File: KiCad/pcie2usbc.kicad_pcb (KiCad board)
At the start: 4 copper layers, 64.5 x 37.3 mm, 70 parts, among them J1 Bus_PCI_Express_x4, J2 Conn_02x05_Top_Bottom, J3 USB-C-MLX, J4 USB-C-MLX

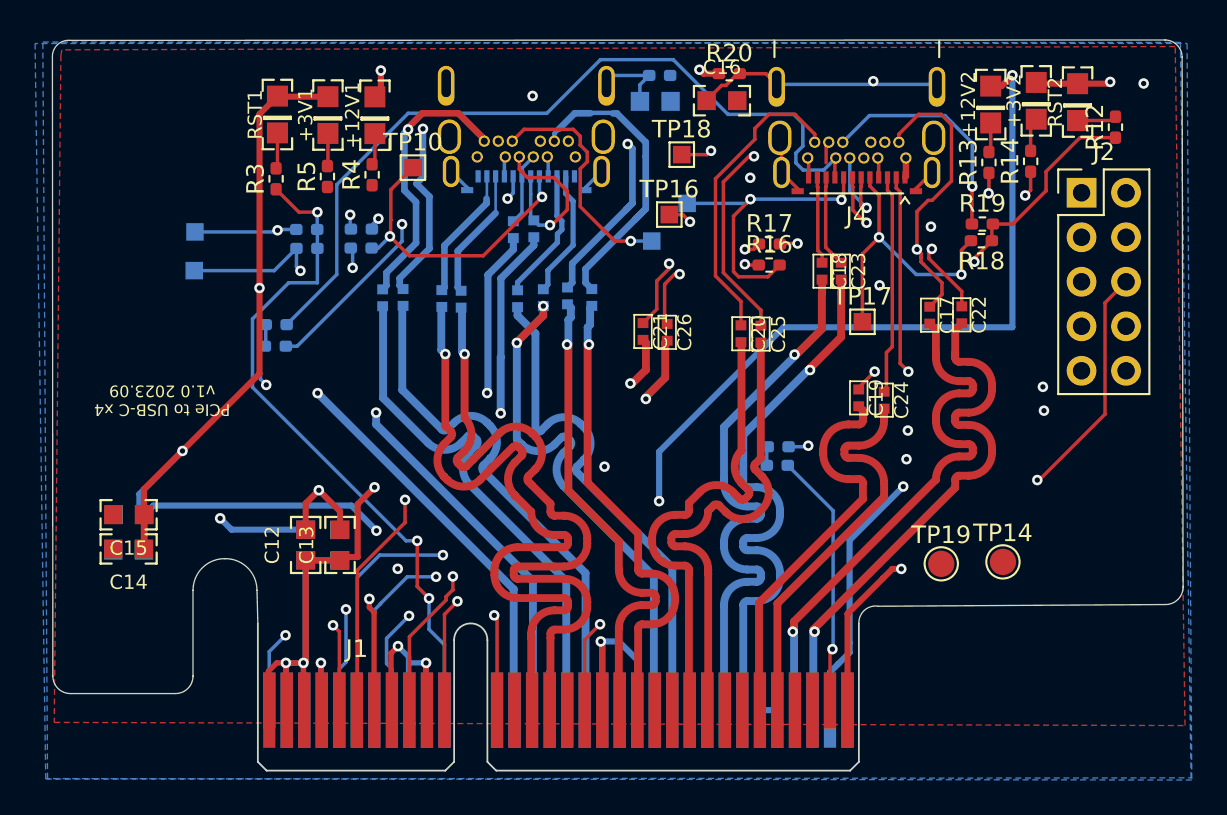
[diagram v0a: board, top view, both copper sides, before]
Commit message: Final rework
Layout completed finally
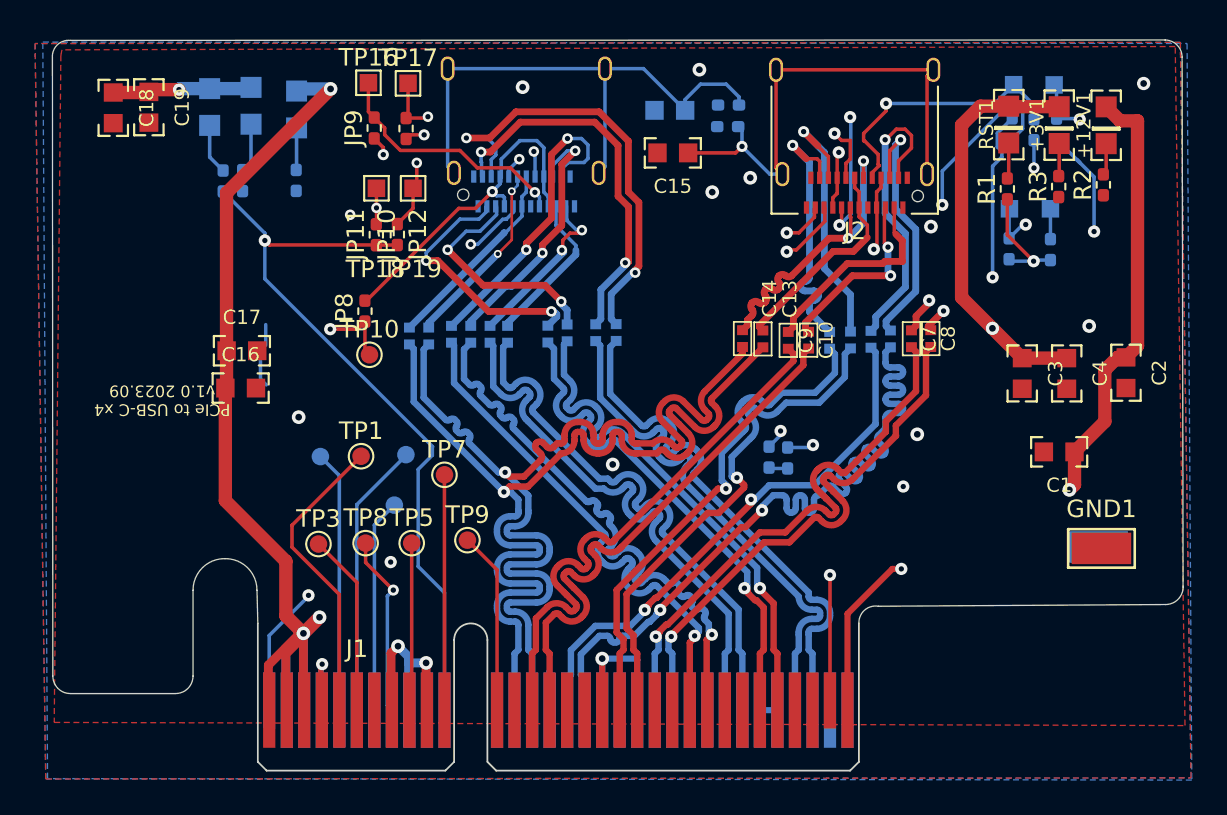
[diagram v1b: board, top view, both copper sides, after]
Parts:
- removed J4: USB-C-MLX, Connector_USB:USB_C_Receptacle_CNCTech_C-ARA1-AK51X
- removed R16, R17, R18, R19: 0, Resistor_SMD:R_0402_1005Metric_Pad0.72x0.64mm_HandSolder
- removed R20: 100k, Resistor_SMD:R_0402_1005Metric_Pad0.72x0.64mm_HandSolder
- added GND1: TestPoint, TestPoint:TestPoint_Keystone_5015_Micro-Minature, F.Cu at (190.7, 104.2)
- added JP3: 0, Resistor_SMD:R_0402_1005Metric_Pad0.72x0.64mm_HandSolder, B.Cu at (185.6, 80.3)
- added JP4: 0, Resistor_SMD:R_0402_1005Metric_Pad0.72x0.64mm_HandSolder, B.Cu at (188.1, 80.3)
- added JP5: 0, Resistor_SMD:R_0402_1005Metric_Pad0.72x0.64mm_HandSolder, B.Cu at (186.8, 80.3)
- added JP6: 0, Resistor_SMD:R_0402_1005Metric_Pad0.72x0.64mm_HandSolder, B.Cu at (187.8, 87.2)
- added JP7: 0, Resistor_SMD:R_0402_1005Metric_Pad0.72x0.64mm_HandSolder, B.Cu at (185.4, 87.1)
- added TP1: TestPoint_Small, TestPoint:TestPoint_Pad_D1.0mm, F.Cu at (148.4, 99.0)
- added TP2: TestPoint_Small, TestPoint:TestPoint_Pad_D1.0mm, B.Cu at (146.1, 99.0)
- added TP3: TestPoint_Small, TestPoint:TestPoint_Pad_D1.0mm, F.Cu at (146.0, 104.0)
- added TP4: TestPoint_Small, TestPoint:TestPoint_Pad_D1.0mm, B.Cu at (151.0, 98.9)
- added TP5: TestPoint_Small, TestPoint:TestPoint_Pad_D1.0mm, F.Cu at (151.3, 103.9)
- added TP6: TestPoint_Small, TestPoint:TestPoint_Pad_D1.0mm, B.Cu at (150.3, 101.8)
- added TP7: TestPoint_Small, TestPoint:TestPoint_Pad_D1.0mm, F.Cu at (153.2, 100.0)
- added TP8: TestPoint_Small, TestPoint:TestPoint_Pad_D1.0mm, F.Cu at (148.7, 103.9)
- added TP9: TestPoint_Small, TestPoint:TestPoint_Pad_D1.0mm, F.Cu at (154.5, 103.8)
- +12V2, +3V2, C20, C21, C22, C23, C24, C25, C26, RST2: moved to B.Cu
- C1: value 100n -> 1u; moved to F.Cu
- C10, C7, C8, C9: moved to F.Cu
- C12: value 1u -> 100n; footprint pcie2usbc:C0603K -> pcie2usbc:C0402; moved to B.Cu
- C13, C28: footprint pcie2usbc:C0603K -> pcie2usbc:C0402
- C14, C27, C29: value 1u -> 100n; footprint pcie2usbc:C0603K -> pcie2usbc:C0402
- C16: value 100n -> 1u
- C17, C19: footprint pcie2usbc:C0402 -> pcie2usbc:C0603K
- C18: value 100n -> 1u; footprint pcie2usbc:C0402 -> pcie2usbc:C0603K
- C2, C4: footprint pcie2usbc:C0402 -> pcie2usbc:C0603K; moved to F.Cu
- C3: value 100n -> 1u; footprint pcie2usbc:C0402 -> pcie2usbc:C0603K; moved to F.Cu
- J2: value Conn_02x05_Top_Bottom -> USB-C-MLX; footprint Connector_PinHeader_2.54mm:PinHeader_2x05_P2.54mm_Vertical -> Connector_USB:USB_C_Receptacle_Amphenol_12401610E4-2A
- J3: footprint Connector_USB:USB_C_Receptacle_CNCTech_C-ARA1-AK51X -> Connector_USB:USB_C_Receptacle_Amphenol_12401610E4-2A
- JP10: renamed from R12; value 2.2k -> 0
- JP11: renamed from R13; value 10k -> 0
- JP12: renamed from R14; value 2.2k -> 0
- JP8: renamed from R10; moved to F.Cu
- JP9: renamed from R11; value 100k -> 0; moved to F.Cu
- R4: renamed from R6; value 0 -> 100k
- R5: renamed from R7; value 0 -> 2.2k
- R6: renamed from R8; value 0 -> 10k
- R7: renamed from R9; value 0 -> 2.2k
- R8: renamed from R15; value 0 -> 100k
- TP10: value TestPoint -> TestPoint_Small; footprint TestPoint:TestPoint_Pad_1.0x1.0mm -> TestPoint:TestPoint_Pad_D1.0mm
- TP14: value TPTP38X20 -> TestPoint; footprint TestPoint:TestPoint_Pad_D1.5mm -> TestPoint:TestPoint_Pad_1.0x1.0mm; moved to B.Cu
- TP15: footprint TestPoint:TestPoint_Pad_1.0x1.0mm -> TestPoint:TestPoint_Keystone_5015_Micro-Minature
- TP19: value TPTP38X20 -> TestPoint; footprint TestPoint:TestPoint_Pad_D1.5mm -> TestPoint:TestPoint_Pad_1.0x1.0mm
- moved RST2 49.5 mm to (139.8, 79.0)
- moved TP13 49.0 mm to (187.8, 84.8), turned to -90 degrees
- moved TP12 47.5 mm to (185.7, 77.8), turned to -90 degrees
- moved +3V2 44.8 mm to (142.2, 79.0)
- moved C19 43.8 mm to (136.3, 79.0)
- moved C2 42.6 mm to (192.1, 94.2)
- moved +12V1 41.7 mm to (191.0, 80.1)
- moved R2 41.7 mm to (190.8, 83.5)
- moved RST1 41.7 mm to (185.4, 80.0)
- moved +3V1 41.7 mm to (188.3, 80.1)
- moved R1 41.7 mm to (185.3, 83.7)
- moved R3 41.7 mm to (188.2, 83.6)
- moved C18 41.5 mm to (134.3, 79.1)
- moved JP10 40.5 mm to (151.0, 80.3)
- moved +12V2 39.6 mm to (144.8, 79.2)
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- renumbered R1 to JP1, R2 to JP2, R3 to R1, R4 to R2, R5 to R3
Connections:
- C1 pad 1: Net-(C1-Pad1) -> +12V
- C10 pad 1: /USB-C Lane1+2/TX2_N -> /USB-C Lane1+2/TX1_N
- C10 pad 2: /PET1_N -> /PET0_N
- C11 pad 1: /USB-C Lane1+2/D_N -> /USB-C Lane1+2/TX2_P
- C11 pad 2: /REFCLK_N -> /PET1_P
- C12 pad 1: +12V -> /USB-C Lane1+2/TX2_N
- C12 pad 2: GND -> /PET1_N
- C13 pad 1: +12V -> /USB-C Lane1+2/D_P
- C13 pad 2: GND -> /REFCLK_P
- C14 pad 1: +3V3 -> /USB-C Lane1+2/D_N
- C14 pad 2: GND -> /REFCLK_N
- C15 pad 1: +3V3 -> Net-(J2-SHIELD)
- C16 pad 1: Net-(C16-Pad1) -> +12V
- C17 pad 1: /USB-C Lane3+4/RX1_P -> +12V
- C17 pad 2: /PER3_P -> GND
- C18 pad 1: /USB-C Lane3+4/RX2_P -> +3V3
- C18 pad 2: /PER2_P -> GND
- C19 pad 1: /USB-C Lane3+4/TX1_P -> +3V3
- C19 pad 2: /PET3_P -> GND
- C2 pad 1: /USB-C Lane1+2/RX1_P -> +12V
- C2 pad 2: /PER0_P -> GND
- C20 pad 1: /USB-C Lane3+4/TX2_P -> /USB-C Lane3+4/RX1_P
- C20 pad 2: /PET2_P -> /PER3_P
- C21 pad 1: /USB-C Lane3+4/D_P -> /USB-C Lane3+4/RX1_N
- C21 pad 2: /REFCLK_P -> /PER3_N
- C22 pad 1: /USB-C Lane3+4/RX1_N -> /USB-C Lane3+4/RX2_P
- C22 pad 2: /PER3_N -> /PER2_P
- C24 pad 1: /USB-C Lane3+4/TX1_N -> /USB-C Lane3+4/TX1_P
- C24 pad 2: /PET3_N -> /PET3_P
- C25 pad 1: /USB-C Lane3+4/TX2_N -> /USB-C Lane3+4/TX1_N
- C25 pad 2: /PET2_N -> /PET3_N
- C26 pad 1: /USB-C Lane3+4/D_N -> /USB-C Lane3+4/TX2_P
- C26 pad 2: /REFCLK_N -> /PET2_P
- C27 pad 1: +12V -> /USB-C Lane3+4/TX2_N
- C27 pad 2: GND -> /PET2_N
- C28 pad 1: +12V -> /USB-C Lane3+4/D_P
- C28 pad 2: GND -> /REFCLK_P
- C29 pad 1: +3V3 -> /USB-C Lane3+4/D_N
- C29 pad 2: GND -> /REFCLK_N
- C3 pad 1: /USB-C Lane1+2/RX2_P -> +3V3
- C3 pad 2: /PER1_P -> GND
- C30 pad 1: +3V3 -> Net-(J3-SHIELD)
- C4 pad 1: /USB-C Lane1+2/TX1_P -> +3V3
- C4 pad 2: /PET0_P -> GND
- C5 pad 1: /USB-C Lane1+2/TX2_P -> /USB-C Lane1+2/RX1_P
- C5 pad 2: /PET1_P -> /PER0_P
- C6 pad 1: /USB-C Lane1+2/D_P -> /USB-C Lane1+2/RX1_N
- C6 pad 2: /REFCLK_P -> /PER0_N
- C7 pad 1: /USB-C Lane1+2/RX1_N -> /USB-C Lane1+2/RX2_P
- C7 pad 2: /PER0_N -> /PER1_P
- C9 pad 1: /USB-C Lane1+2/TX1_N -> /USB-C Lane1+2/TX1_P
- C9 pad 2: /PET0_N -> /PET0_P
- J1 pad B17: /PRSNT2 -> unconnected-(J1-~{PRSNT2}-PadB17)
- J3 pad A10: /USB-C Lane1+2/RX2_N -> /USB-C Lane3+4/RX2_N
- J3 pad A11: /USB-C Lane1+2/RX2_P -> /USB-C Lane3+4/RX2_P
- J3 pad A2: /USB-C Lane1+2/TX1_P -> /USB-C Lane3+4/TX1_P
- J3 pad A3: /USB-C Lane1+2/TX1_N -> /USB-C Lane3+4/TX1_N
- J3 pad A4: /USB-C Lane1+2/VBUS -> /USB-C Lane3+4/VBUS
- J3 pad A5: /USB-C Lane1+2/CC1 -> /USB-C Lane3+4/CC1
- J3 pad A6: /USB-C Lane1+2/D_P -> /USB-C Lane3+4/D_P
- J3 pad A7: /USB-C Lane1+2/D_N -> /USB-C Lane3+4/D_N
- J3 pad A8: /USB-C Lane1+2/SBU1 -> /USB-C Lane3+4/SBU1
- J3 pad A9: /USB-C Lane1+2/VBUS -> /USB-C Lane3+4/VBUS
- J3 pad B10: /USB-C Lane1+2/RX1_N -> /USB-C Lane3+4/RX1_N
- J3 pad B11: /USB-C Lane1+2/RX1_P -> /USB-C Lane3+4/RX1_P
- J3 pad B2: /USB-C Lane1+2/TX2_P -> /USB-C Lane3+4/TX2_P
- J3 pad B3: /USB-C Lane1+2/TX2_N -> /USB-C Lane3+4/TX2_N
- J3 pad B4: /USB-C Lane1+2/VBUS -> /USB-C Lane3+4/VBUS
- J3 pad B5: /USB-C Lane1+2/CC2 -> /USB-C Lane3+4/CC2
- J3 pad B6: /USB-C Lane1+2/D_P -> /USB-C Lane3+4/D_P
- J3 pad B7: /USB-C Lane1+2/D_N -> /USB-C Lane3+4/D_N
- J3 pad B8: /USB-C Lane1+2/SBU2 -> /USB-C Lane3+4/SBU2
- J3 pad B9: /USB-C Lane1+2/VBUS -> /USB-C Lane3+4/VBUS
- J3 pad S1: Net-(C1-Pad1) -> Net-(J3-SHIELD)
- JP1 pad 1: /PRSNT_SEL -> /PRSNT1
- JP1 pad 2: /PRSNT2 -> /PRSNT_SEL
- JP10 pad 2: Net-(R12-Pad2) -> /USB-C Lane3+4/SBU2
- JP11 pad 1: GND -> /PERST_N
- JP11 pad 2: Net-(+12V2-PadC) -> /USB-C Lane3+4/CC1
- JP12 pad 1: GND -> /USB-C Lane3+4/CC2
- JP12 pad 2: Net-(+3V2-PadC) -> /PERST_N
- JP2 pad 1: /PRSNT1 -> /PRSNT_SEL
- JP2 pad 2: /PRSNT_SEL -> /PRSNT2
- JP8 pad 1: /USB-C Lane1+2/CC2 -> /PERST_N
- JP8 pad 2: /PERST_N -> /USB-C Lane3+4/VBUS
- JP9 pad 1: GND -> /PRSNT2_N
- JP9 pad 2: Net-(C1-Pad1) -> /USB-C Lane3+4/SBU1
- R4 pad 1: /VBUS_H -> GND
- R4 pad 2: /USB-C Lane1+2/VBUS -> Net-(J2-SHIELD)
- R5 pad 1: /PRSNT2_N -> /PERST_N
- R5 pad 2: /USB-C Lane1+2/SBU1 -> Net-(R5-Pad2)
- R6 pad 1: /PRSNT1_N -> GND
- R6 pad 2: /USB-C Lane1+2/SBU2 -> Net-(+12V2-PadC)
- R7 pad 1: /PERST_N -> GND
- R7 pad 2: /USB-C Lane1+2/CC1 -> Net-(+3V2-PadC)
- R8 pad 1: /VBUS_H -> GND
- R8 pad 2: /USB-C Lane3+4/VBUS -> Net-(J3-SHIELD)
- RST2 pad C: Net-(R12-Pad2) -> Net-(R5-Pad2)
- TP10 pad 1: /USB-C Lane1+2/SBU1 -> /PERST_N
- TP11 pad 1: /USB-C Lane1+2/SBU2 -> /PERST_N
- TP12 pad 1: /USB-C Lane1+2/CC1 -> /USB-C Lane1+2/SBU2
- TP13 pad 1: /USB-C Lane1+2/CC2 -> /USB-C Lane1+2/CC1
- TP14 pad 1: (no net) -> /USB-C Lane1+2/CC2
- TP15 pad 1: /USB-C Lane3+4/SBU1 -> GND
- TP16 pad 1: /USB-C Lane3+4/SBU2 -> /USB-C Lane3+4/SBU1
- TP17 pad 1: /USB-C Lane3+4/CC1 -> /USB-C Lane3+4/SBU2
- TP18 pad 1: /USB-C Lane3+4/CC2 -> /USB-C Lane3+4/CC1
- TP19 pad 1: (no net) -> /USB-C Lane3+4/CC2
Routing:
- net /PERST_N: track 89.5 -> 230.0 mm, vias 4 -> 9
- net /VBUS_H: track 55.2 -> 0.00 mm, vias 2 -> 0
- net /SMDAT: track 63.3 -> 10.4 mm, vias 1 -> 0
- net /TCK: track 63.4 -> 14.9 mm, vias 3 -> 0
- net /SMCLK: track 64.9 -> 17.2 mm, vias 2 -> 0
- net Net-(J3-SHIELD): track 0.00 -> 45.6 mm
- net /TDO: track 57.3 -> 12.2 mm, vias 1 -> 0
- net /TRST_N: track 52.6 -> 9.58 mm, vias 1 -> 0
- net /TMS: track 51.7 -> 10.4 mm, vias 2 -> 1
- net /TDI: track 57.0 -> 15.7 mm, vias 1 -> 0
- net GND: track 69.3 -> 109.9 mm, vias 17 -> 16
- net /WAKE_N: track 53.4 -> 13.4 mm, vias 1 -> 0
- net /USB-C Lane3+4/SBU2: track 48.8 -> 10.8 mm
- net /CLKREQ_N: track 46.8 -> 10.4 mm, vias 1 -> 0
- net Net-(C16-Pad1): track 33.1 -> 0.00 mm, vias 1 -> 0
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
